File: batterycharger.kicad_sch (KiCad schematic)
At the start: 29 parts, among them J1 Barrel_Jack, U1 LT3652EMSE, U2 INA234AxYBJ

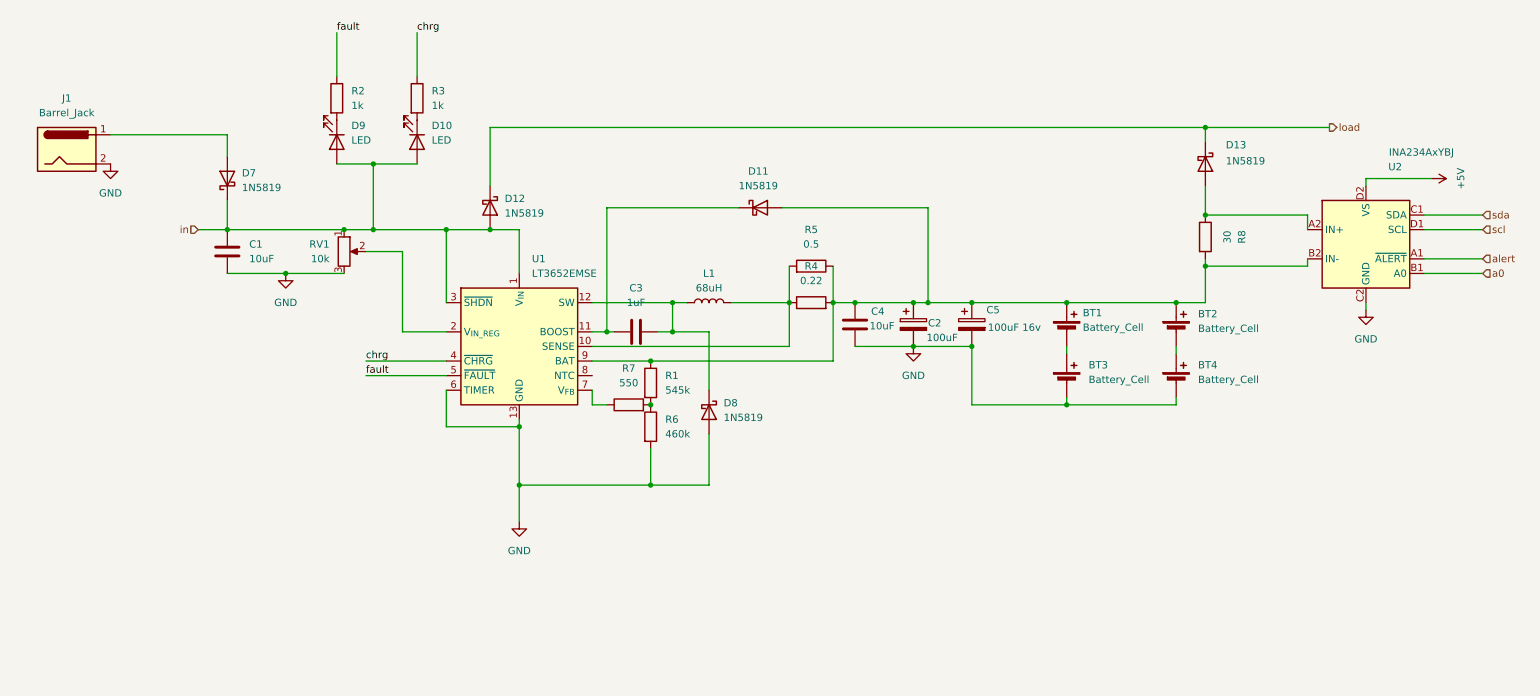
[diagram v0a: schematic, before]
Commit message: new design
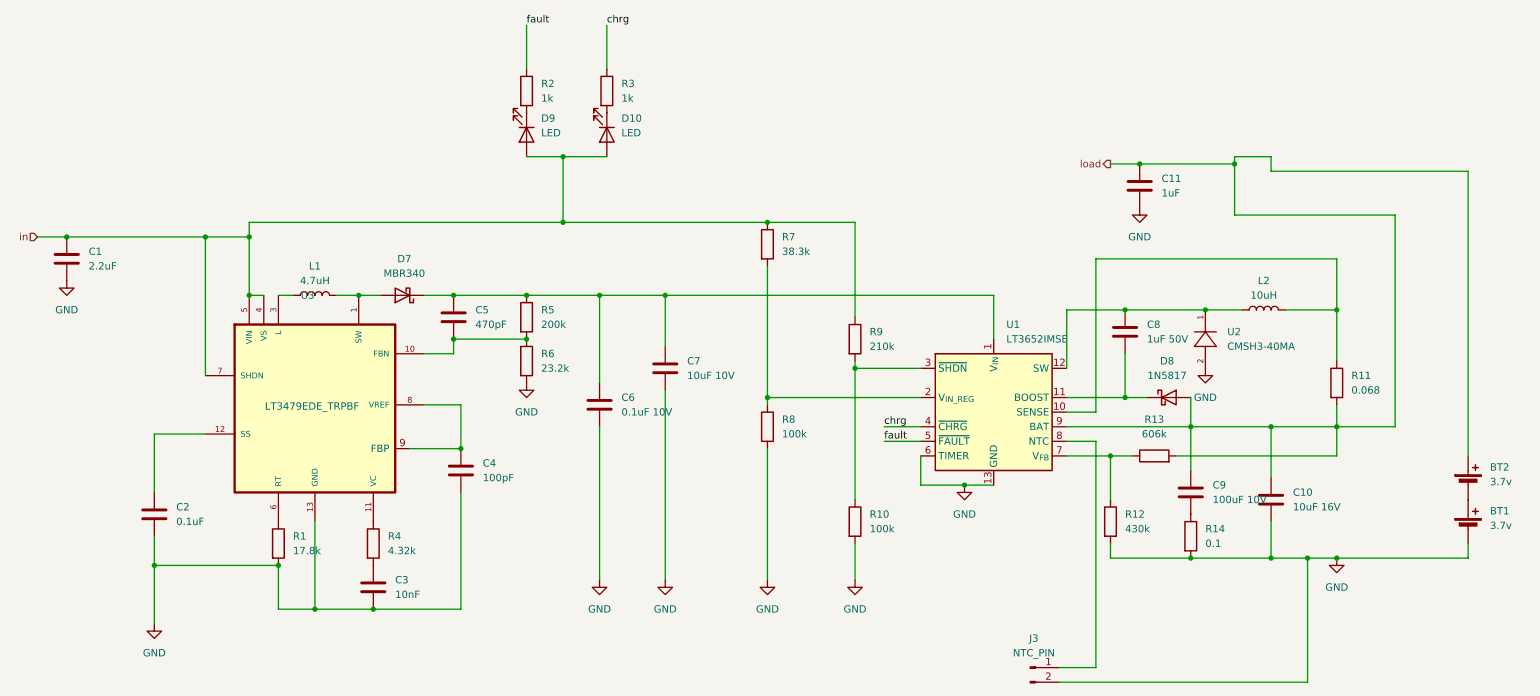
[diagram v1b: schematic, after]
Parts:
- removed BT3, BT4: Battery_Cell, Battery:BatteryHolder_Keystone_1042_1x18650, symbol Device:Battery_Cell
- removed C2: 100uF, Capacitor_THT:CP_Radial_D6.3mm_P2.50mm, symbol Device:C_Polarized
- removed C5: 100uF 16v, Capacitor_THT:CP_Radial_D6.3mm_P2.50mm, symbol Device:C_Polarized
- removed D11, D12, D13, D7, D8: 1N5819, Diode_THT:D_DO-41_SOD81_P10.16mm_Horizontal, symbol Diode:1N5819
- removed J1: Barrel_Jack, Connector_BarrelJack:BarrelJack_SwitchcraftConxall_RAPC10U_Horizontal, symbol Connector:Barrel_Jack
- removed RV1: 10k, Potentiometer_THT:Potentiometer_Bourns_3386P_Vertical, symbol Device:R_Potentiometer
- removed U1: LT3652EMSE, Package_SO:MSOP-12-1EP_3x4mm_P0.65mm_EP1.65x2.85mm, symbol Battery_Management:LT3652EMSE
- removed U2: INA234AxYBJ, Package_BGA:Texas_DSBGA-8_0.705x1.468mm_Layout2x4_P0.4mm, symbol Analog_ADC:INA234AxYBJ
- added C10: 10uF 16V, Capacitor_SMD:C_0805_2012Metric_Pad1.18x1.45mm_HandSolder, symbol Device:C
- added C11: 1uF, Capacitor_SMD:C_0603_1608Metric_Pad1.08x0.95mm_HandSolder, symbol Device:C
- added C2: 0.1uF, Capacitor_SMD:C_0603_1608Metric_Pad1.08x0.95mm_HandSolder, symbol Device:C
- added C5: 470pF, Capacitor_SMD:C_0603_1608Metric_Pad1.08x0.95mm_HandSolder, symbol Device:C
- added C6: 0.1uF 10V, Capacitor_SMD:C_0201_0603Metric_Pad0.64x0.40mm_HandSolder, symbol Device:C
- added C7: 10uF 10V, Capacitor_SMD:C_0805_2012Metric_Pad1.18x1.45mm_HandSolder, symbol Device:C
- added C8: 1uF 50V, Capacitor_SMD:C_0402_1005Metric_Pad0.74x0.62mm_HandSolder, symbol Device:C
- added C9: 100uF 10V, Capacitor_THT:C_Radial_D5.0mm_H11.0mm_P2.00mm, symbol Device:C
- added D7: MBR340, Diode_THT:D_DO-201AD_P15.24mm_Horizontal, symbol Diode:MBR340
- added D8: 1N5817, Diode_THT:D_DO-41_SOD81_P10.16mm_Horizontal, symbol Diode:1N5817
- added J3: NTC_PIN, Connector_PinHeader_2.54mm:PinHeader_1x02_P2.54mm_Vertical, symbol Connector:Conn_01x02_Pin
- added L2: 10uH, Inductor_SMD:L_2512_6332Metric_Pad1.52x3.35mm_HandSolder, symbol Device:L
- added R10: 100k, Resistor_THT:R_Axial_DIN0207_L6.3mm_D2.5mm_P15.24mm_Horizontal, symbol Device:R
- added R11: 0.068, Resistor_THT:R_Axial_DIN0207_L6.3mm_D2.5mm_P15.24mm_Horizontal, symbol Device:R
- added R12: 430k, Resistor_THT:R_Axial_DIN0207_L6.3mm_D2.5mm_P15.24mm_Horizontal, symbol Device:R
- added R13: 606k, Resistor_THT:R_Axial_DIN0207_L6.3mm_D2.5mm_P15.24mm_Horizontal, symbol Device:R
- added R14: 0.1, Resistor_THT:R_Axial_DIN0207_L6.3mm_D2.5mm_P15.24mm_Horizontal, symbol Device:R
- added R9: 210k, Resistor_THT:R_Axial_DIN0207_L6.3mm_D2.5mm_P15.24mm_Horizontal, symbol Device:R
- added U1: LT3652IMSE, Package_SO:MSOP-12-1EP_3x4mm_P0.65mm_EP1.65x2.85mm, symbol Battery_Management:LT3652IMSE
- added U2: CMSH3-40MA, CMSH3-40MA:SMA, symbol CMSH3-40MA:CMSH3-40MA
- added U3: LT3479EDE_TRPBF, LT3479EDE_TRPBF:DFN-14_DE, symbol LT3479EDE_TRPBF:LT3479EDE_TRPBF
- BT1, BT2: value Battery_Cell -> 3.7v
- C1: value 10uF -> 2.2uF; footprint Capacitor_THT:C_Disc_D5.1mm_W3.2mm_P5.00mm -> Capacitor_SMD:C_0402_1005Metric_Pad0.74x0.62mm_HandSolder
- C3: value 1uF -> 10nF; footprint Capacitor_THT:C_Disc_D5.0mm_W2.5mm_P2.50mm -> Capacitor_SMD:C_0805_2012Metric_Pad1.18x1.45mm_HandSolder
- C4: value 10uF -> 100pF; footprint Capacitor_THT:C_Disc_D5.1mm_W3.2mm_P5.00mm -> Capacitor_SMD:C_0402_1005Metric_Pad0.74x0.62mm_HandSolder
- D10, D9: footprint LED_THT:LED_Rectangular_W3.0mm_H2.0mm -> LED_THT:LED_D5.0mm
- L1: value 68uH -> 4.7uH; footprint Inductor_THT:L_Axial_L5.0mm_D3.6mm_P10.00mm_Horizontal_Murata_BL01RN1A2A2 -> Inductor_THT:L_Radial_D8.7mm_P5.00mm_Fastron_07HCP
- R1: value 545k -> 17.8k; footprint Resistor_THT:R_Axial_DIN0204_L3.6mm_D1.6mm_P5.08mm_Horizontal -> Resistor_THT:R_Axial_DIN0207_L6.3mm_D2.5mm_P15.24mm_Horizontal
- R2, R3: footprint Resistor_THT:R_Axial_DIN0204_L3.6mm_D1.6mm_P5.08mm_Horizontal -> Resistor_THT:R_Axial_DIN0207_L6.3mm_D2.5mm_P15.24mm_Horizontal
- R4: value 0.22 -> 4.32k; footprint Resistor_THT:R_Axial_DIN0204_L3.6mm_D1.6mm_P5.08mm_Horizontal -> Resistor_THT:R_Axial_DIN0207_L6.3mm_D2.5mm_P15.24mm_Horizontal
- R5: value 0.5 -> 200k; footprint Resistor_THT:R_Axial_DIN0204_L3.6mm_D1.6mm_P5.08mm_Horizontal -> Resistor_THT:R_Axial_DIN0207_L6.3mm_D2.5mm_P15.24mm_Horizontal
- R6: value 460k -> 23.2k; footprint Resistor_THT:R_Axial_DIN0204_L3.6mm_D1.6mm_P5.08mm_Horizontal -> Resistor_THT:R_Axial_DIN0207_L6.3mm_D2.5mm_P15.24mm_Horizontal
- R7: value 550 -> 38.3k; footprint Resistor_THT:R_Axial_DIN0204_L3.6mm_D1.6mm_P5.08mm_Horizontal -> Resistor_THT:R_Axial_DIN0207_L6.3mm_D2.5mm_P15.24mm_Horizontal
- R8: value 30 -> 100k; footprint Resistor_THT:R_Axial_DIN0204_L3.6mm_D1.6mm_P5.08mm_Horizontal -> Resistor_THT:R_Axial_DIN0207_L6.3mm_D2.5mm_P15.24mm_Horizontal
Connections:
- net GND: now also BT1.2 (-), C3.2, R1.2, R8.2, C10.2, C11.2, C2.2, C6.2, C7.2, J3.2 (Pin_2), R10.2, R12.2, R14.2, U1.13 (GND), U1.6 (TIMER), U2.2, U3.13 (GND)
- net chrg: now also U1.4 (~{CHRG})
- net fault: now also U1.5 (~{FAULT})
- net in: now also R7.1, R9.1, U3.4 (VS), U3.5 (VIN), U3.7 (SHDN)
- net load: now also BT2.1 (+), C10.1, C11.1, C9.1, D8.2 (A), R11.2, R13.2, U1.9 (BAT)
- net at C3.1: now also R4.2
- net at L1.1: now also U3.3 (L); no longer C3.2
- net at R8.1: now also R7.2, U1.2 (V_{IN_REG})
- net at BT2.2 (-): now also BT1.1 (+)
- new net: C5.1, C6.1, C7.1, D7.1 (K), R5.1, U1.1 (V_{IN})
- new net: D7.2 (A), L1.2, U3.1 (SW)
- new net: C5.2, R5.2, R6.1, U3.10 (FBN)
- new net: C8.1, L2.1, U1.12 (SW), U2.1
- new net: L2.2, R11.1, U1.10 (SENSE)
- new net: C8.2, D8.1 (K), U1.11 (BOOST)
- new net: R10.1, R9.2, U1.3 (~{SHDN})
- new net: R12.1, R13.1, U1.7 (V_{FB})
- new net: J3.1 (Pin_1), U1.8 (NTC)
- new net: C9.2, R14.1
- new net: R4.1, U3.11 (VC)
- new net: C2.1, U3.12 (SS)
- new net: R1.1, U3.6 (RT)
- new net: C4.1, U3.8 (VREF), U3.9 (FBP)
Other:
- moved on the sheet: D10, D9, R2, R3

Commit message: fixed
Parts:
- U3: footprint LT3479EDE_TRPBF:DFN-14_DE -> footprints:DFN-14_DE_LIT
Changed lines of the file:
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@@
 			)
 		)
-		(property "Footprint" "LT3479EDE_TRPBF:DFN-14_DE"
+		(property "Footprint" "footprints:DFN-14_DE_LIT"
 			(at 58.928 141.732 0)
 			(effects
